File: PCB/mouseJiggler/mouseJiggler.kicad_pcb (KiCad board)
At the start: 2 copper layers, 2 parts, among them J1 USB_A, J2 USB_A

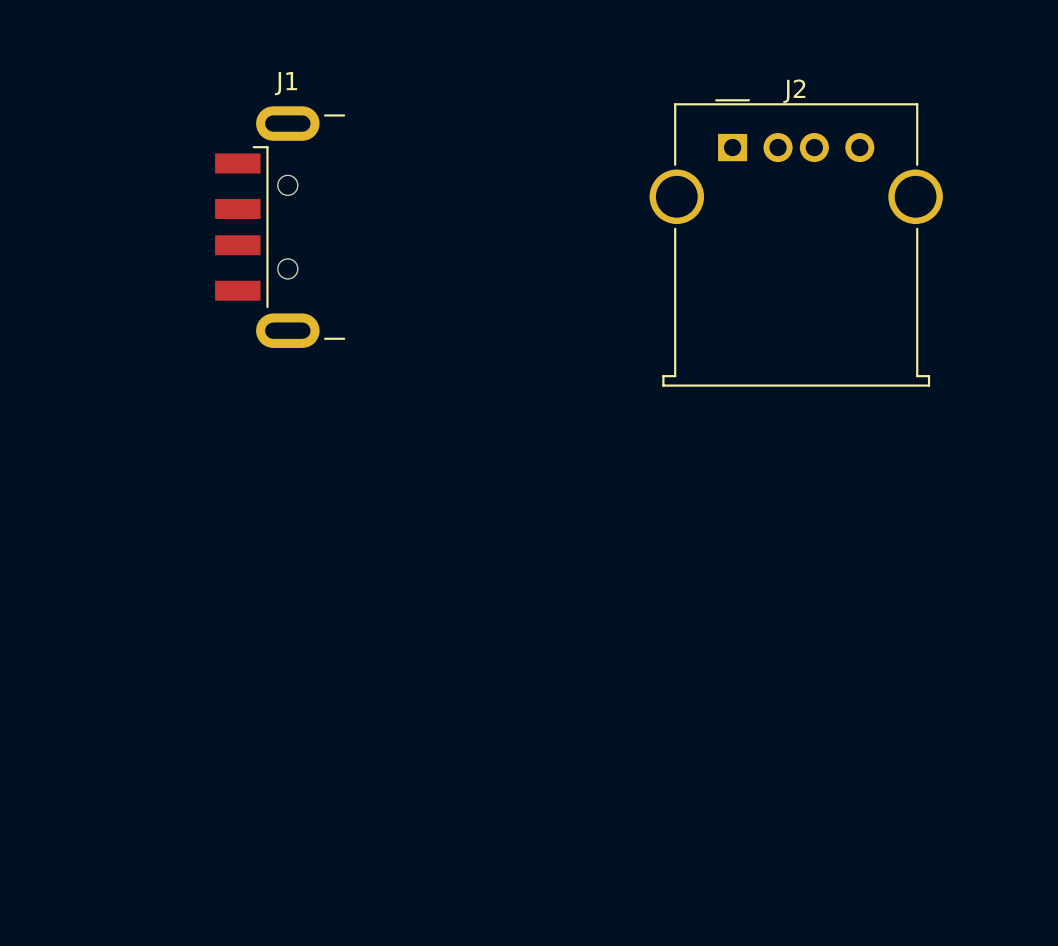
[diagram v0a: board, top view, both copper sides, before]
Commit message: Updated schematic
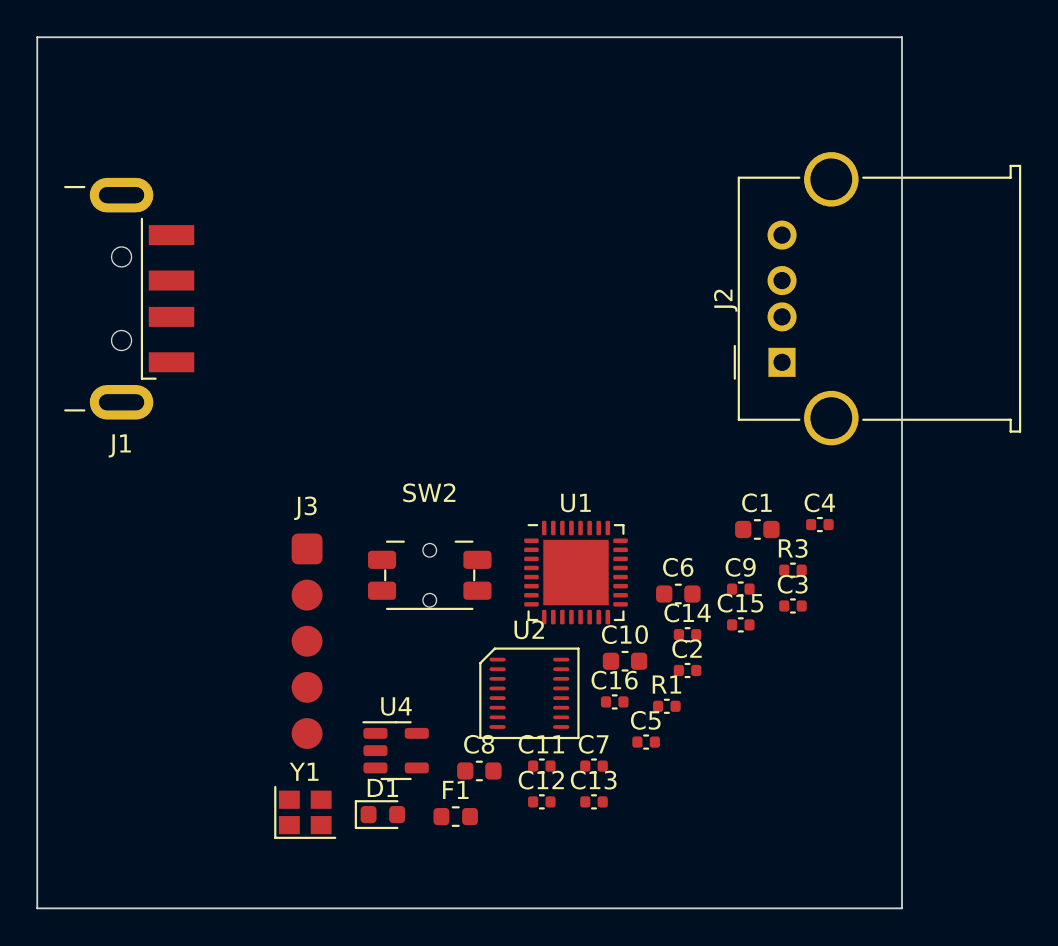
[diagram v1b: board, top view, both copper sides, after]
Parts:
- added C1: 10u, Capacitor_SMD:C_0603_1608Metric, F.Cu at (133.2, 113.9)
- added C10: 10u, Capacitor_SMD:C_0603_1608Metric, F.Cu at (125.9, 121.2)
- added C11: 10u, Capacitor_SMD:C_0402_1005Metric, F.Cu at (121.3, 127.0)
- added C12: 10u, Capacitor_SMD:C_0402_1005Metric, F.Cu at (121.3, 128.9)
- added C13: 100n, Capacitor_SMD:C_0402_1005Metric, F.Cu at (124.2, 128.9)
- added C14: 30p, Capacitor_SMD:C_0402_1005Metric, F.Cu at (129.3, 119.7)
- added C15: 1u, Capacitor_SMD:C_0402_1005Metric, F.Cu at (132.3, 119.2)
- added C16: 1u, Capacitor_SMD:C_0402_1005Metric, F.Cu at (125.3, 123.4)
- added C2: 100n, Capacitor_SMD:C_0402_1005Metric, F.Cu at (129.3, 121.7)
- added C3: 1u, Capacitor_SMD:C_0402_1005Metric, F.Cu at (135.2, 118.1)
- added C4: 100n, Capacitor_SMD:C_0402_1005Metric, F.Cu at (136.6, 113.7)
- added C5: 100n, Capacitor_SMD:C_0402_1005Metric, F.Cu at (127.1, 125.6)
- added C6: 10u, Capacitor_SMD:C_0603_1608Metric, F.Cu at (128.8, 117.5)
- added C7: 30p, Capacitor_SMD:C_0402_1005Metric, F.Cu at (124.2, 127.0)
- added C8: 10u, Capacitor_SMD:C_0603_1608Metric, F.Cu at (117.9, 127.2)
- added C9: 100n, Capacitor_SMD:C_0402_1005Metric, F.Cu at (132.3, 117.2)
- added D1: LED, LED_SMD:LED_0603_1608Metric, F.Cu at (112.6, 129.6)
- added F1: 500mA, josh-passives-smt:Fuse_0603_1608Metric, F.Cu at (116.6, 129.7)
- added J3: SWD, josh-connectors:5_PIN_SMD_PROG, F.Cu at (108.4, 115.0)
- added R1: 3K3, Capacitor_SMD:C_0402_1005Metric, F.Cu at (128.2, 123.7)
- added R3: 10K, Capacitor_SMD:C_0402_1005Metric, F.Cu at (135.2, 116.2)
- added SW2: SW_Push, josh-buttons-switches:SW_PUSH_EVQPUL_EVQPUC, F.Cu at (115.2, 116.5)
- added U1: ATSAMD21E17A-M, Package_DFN_QFN:QFN-32-1EP_5x5mm_P0.5mm_EP3.6x3.6mm, F.Cu at (123.2, 116.3)
- added U2: SL2.1S, bing-SOIC:SSOP-16_4.6x2.6mm_P0.53, F.Cu at (120.6, 122.6)
- added U4: AP2112K-3.3, Package_TO_SOT_SMD:SOT-23-5, F.Cu at (113.3, 126.1)
- added Y1: 12MHz, Crystal:Crystal_SMD_2520-4Pin_2.5x2.0mm, F.Cu at (108.3, 129.5)
- moved J1 23.3 mm to (91.3, 101.2), turned to 180 degrees
- moved J2 12.1 mm to (134.6, 104.7), turned to 90 degrees
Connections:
- J1 pad 1: unconnected-(J1-Pad1) -> Net-(C10-Pad1)
- J1 pad 2: unconnected-(J1-Pad2) -> /USB_D1-
- J1 pad 3: unconnected-(J1-Pad3) -> /USB_D1+
- J1 pad 4: unconnected-(J1-Pad4) -> GND
- J1 pad 5: unconnected-(J1-Pad5) -> GND
- J2 pad 1: unconnected-(J2-Pad1) -> VBUS
- J2 pad 2: unconnected-(J2-Pad2) -> /USB_D2B-
- J2 pad 3: unconnected-(J2-Pad3) -> /USB_D2B+
- J2 pad 4: unconnected-(J2-Pad4) -> GND
- J2 pad 5: unconnected-(J2-Pad5) -> GND
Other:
- board outline added: 47.6 x 47.9 mm
- copper layers 2 -> 4
